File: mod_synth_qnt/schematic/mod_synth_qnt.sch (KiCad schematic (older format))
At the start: 22 parts

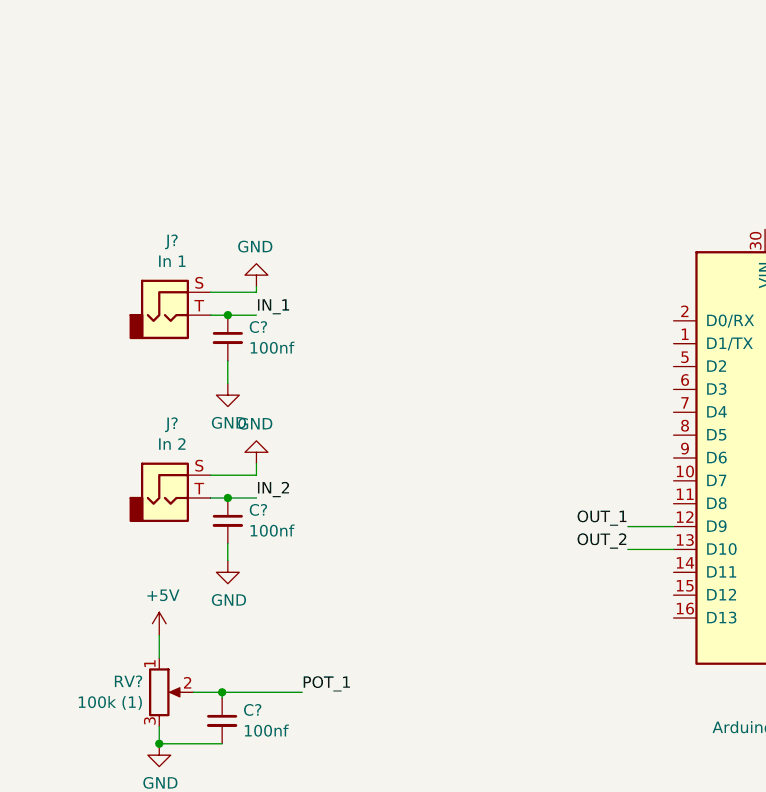
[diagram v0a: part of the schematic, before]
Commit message: Update schematic and code
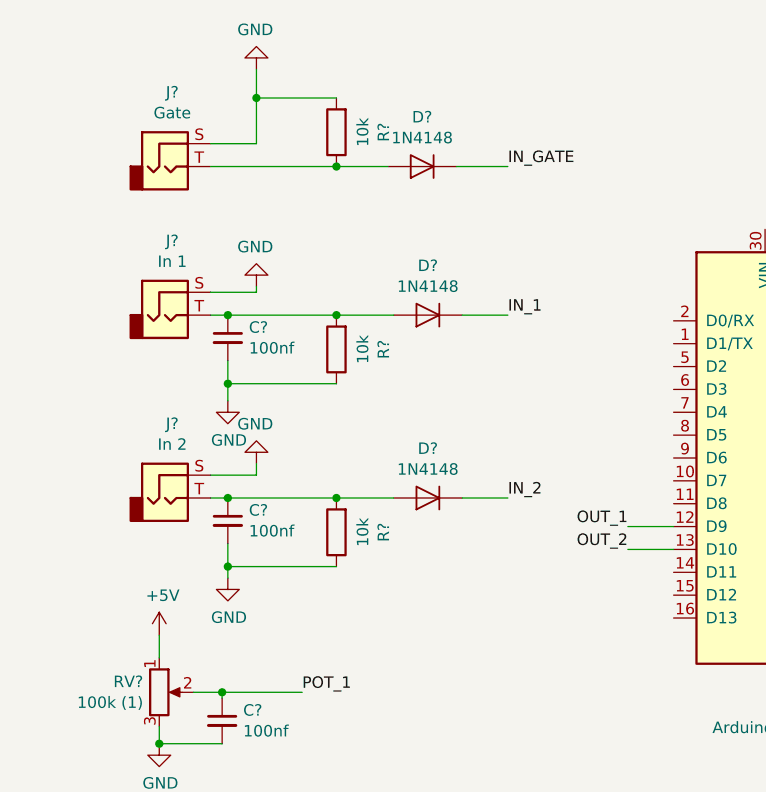
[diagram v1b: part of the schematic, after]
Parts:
- added D? (x3): 1N4148, Diode_THT:D_DO-35_SOD27_P7.62mm_Horizontal, symbol Diode:1N4148
- added J?: Gate, symbol Connector:AudioJack2
- added R? (x3): 10k, symbol Device:R
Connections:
- net GND: now also J?.S, R?.1, R?.1, R?.2
- net IN_1: now also D?.1 (K); no longer C?.1, J?.T
- net IN_2: now also D?.1 (K); no longer C?.1, J?.T
- new net: C?.1, D?.2 (A), J?.T, R?.2 (x2)
- new net: D?.2 (A), J?.T, R?.1
- new net IN_GATE: D?.1 (K)
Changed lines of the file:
@@
 	-1   0    0    -1
 $EndComp
-Text Label 3200 2300 0    50   ~ 0
+Text Label 4300 2300 0    50   ~ 0
 IN_1
-Text Label 3200 3100 0    50   ~ 0
+Text Label 4300 3100 0    50   ~ 0
 IN_2
 $Comp
@@
 Wire Wire Line
 	3200 2950 3200 3000
-Wire Wire Line
-	3200 3100 3075 3100
-Wire Wire Line
-	3200 2300 3075 2300
 Text Label 6225 2925 0    50   ~ 0
 IN_1
@@
 L power:GND #PWR?
 U 1 1 5D619ACB
-P 3075 2600
-F 0 "#PWR?" H 3075 2350 50  0001 C CNN
-F 1 "GND" H 3080 2427 50  0000 C CNN
-F 2 "" H 3075 2600 50  0001 C CNN
-F 3 "" H 3075 2600 50  0001 C CNN
-	1    3075 2600
+P 3075 2675
+F 0 "#PWR?" H 3075 2425 50  0001 C CNN
+F 1 "GND" H 3080 2502 50  0000 C CNN
+F 2 "" H 3075 2675 50  0001 C CNN
+F 3 "" H 3075 2675 50  0001 C CNN
+	1    3075 2675
 	1    0    0    -1
 $EndComp
@@
 L power:GND #PWR?
 U 1 1 5D61A0C8
-P 3075 3375
-F 0 "#PWR?" H 3075 3125 50  0001 C CNN
-F 1 "GND" H 3080 3202 50  0000 C CNN
-F 2 "" H 3075 3375 50  0001 C CNN
-F 3 "" H 3075 3375 50  0001 C CNN
-	1    3075 3375
+P 3075 3450
+F 0 "#PWR?" H 3075 3200 50  0001 C CNN
+F 1 "GND" H 3080 3277 50  0000 C CNN
+F 2 "" H 3075 3450 50  0001 C CNN
+F 3 "" H 3075 3450 50  0001 C CNN
+	1    3075 3450
 	1    0    0    -1
 $EndComp
 Wire Wire Line
 	3075 2600 3075 2500
-Wire Wire Line
-	3075 3300 3075 3375
 $Comp
 L power:GND #PWR?
@@
 NoConn ~ 8275 5300
 NoConn ~ 8275 5200
+$Comp
+L Device:R R?
+U 1 1 5D61316C
+P 3550 2450
+F 0 "R?" V 3343 2450 50  0000 C CNN
+F 1 "10k" V 3434 2450 50  0000 C CNN
+F 2 "" V 3480 2450 50  0001 C CNN
+F 3 "~" H 3550 2450 50  0001 C CNN
+	1    3550 2450
+	-1   0    0    1
+$EndComp
+$Comp
+L Device:R R?
+U 1 1 5D6143B5
+P 3550 3250
+F 0 "R?" V 3343 3250 50  0000 C CNN
+F 1 "10k" V 3434 3250 50  0000 C CNN
+F 2 "" V 3480 3250 50  0001 C CNN
+F 3 "~" H 3550 3250 50  0001 C CNN
+	1    3550 3250
+	-1   0    0    1
+$EndComp
+Wire Wire Line
+	3075 2300 3550 2300
+Wire Wire Line
+	3550 2300 3800 2300
+Connection ~ 3550 2300
+Wire Wire Line
+	3075 3100 3550 3100
+Connection ~ 3550 3100
+Wire Wire Line
+	3550 3100 3800 3100
+Wire Wire Line
+	3550 2600 3075 2600
+Wire Wire Line
+	3075 2600 3075 2675
+Connection ~ 3075 2600
+Wire Wire Line
+	3550 3400 3075 3400
+Wire Wire Line
+	3075 3300 3075 3400
+Connection ~ 3075 3400
+Wire Wire Line
+	3075 3400 3075 3450
+$Comp
+L Connector:AudioJack2 J?
+U 1 1 5D62A188
+P 2800 1650
+F 0 "J?" H 2832 1975 50  0000 C CNN
+F 1 "Gate" H 2832 1884 50  0000 C CNN
+F 2 "" H 2800 1650 50  0001 C CNN
+F 3 "~" H 2800 1650 50  0001 C CNN
+	1    2800 1650
+	1    0    0    -1
+$EndComp
+$Comp
+L power:GND #PWR?
+U 1 1 5D62A425
+P 3200 1225
+F 0 "#PWR?" H 3200 975 50  0001 C CNN
+F 1 "GND" H 3205 1052 50  0000 C CNN
+F 2 "" H 3200 1225 50  0001 C CNN
+F 3 "" H 3200 1225 50  0001 C CNN
+	1    3200 1225
+	-1   0    0    1
+$EndComp
+Wire Wire Line
+	3000 1550 3200 1550
+Text Label 4300 1650 0    50   ~ 0
+IN_GATE
+Wire Wire Line
+	3000 1650 3550 1650
+$Comp
+L Diode:1N4148 D?
+U 1 1 5D630B6B
+P 3925 1650
+F 0 "D?" H 3925 1434 50  0000 C CNN
+F 1 "1N4148" H 3925 1525 50  0000 C CNN
+F 2 "Diode_THT:D_DO-35_SOD27_P7.62mm_Horizontal" H 3925 1475 50  0001 C CNN
+F 3 "https://assets.nexperia.com/documents/data-sheet/1N4148_1N4448.pdf" H 3925 1650 50  0001 C CNN
+	1    3925 1650
+	-1   0    0    1
+$EndComp
+$Comp
+L Diode:1N4148 D?
+U 1 1 5D631B5D
+P 3950 2300
+F 0 "D?" H 3950 2084 50  0000 C CNN
+F 1 "1N4148" H 3950 2175 50  0000 C CNN
+F 2 "Diode_THT:D_DO-35_SOD27_P7.62mm_Horizontal" H 3950 2125 50  0001 C CNN
+F 3 "https://assets.nexperia.com/documents/data-sheet/1N4148_1N4448.pdf" H 3950 2300 50  0001 C CNN
+	1    3950 2300
+	-1   0    0    1
+$EndComp
+$Comp
+L Diode:1N4148 D?
+U 1 1 5D631FDA
+P 3950 3100
+F 0 "D?" H 3950 2884 50  0000 C CNN
+F 1 "1N4148" H 3950 2975 50  0000 C CNN
+F 2 "Diode_THT:D_DO-35_SOD27_P7.62mm_Horizontal" H 3950 2925 50  0001 C CNN
+F 3 "https://assets.nexperia.com/documents/data-sheet/1N4148_1N4448.pdf" H 3950 3100 50  0001 C CNN
+	1    3950 3100
+	-1   0    0    1
+$EndComp
+$Comp
+L Device:R R?
+U 1 1 5D633789
+P 3550 1500
+F 0 "R?" V 3343 1500 50  0000 C CNN
+F 1 "10k" V 3434 1500 50  0000 C CNN
+F 2 "" V 3480 1500 50  0001 C CNN
+F 3 "~" H 3550 1500 50  0001 C CNN
+	1    3550 1500
+	-1   0    0    1
+$EndComp
+Connection ~ 3550 1650
+Wire Wire Line
+	3550 1650 3775 1650
+Wire Wire Line
+	4075 1650 4300 1650
+Wire Wire Line
+	4300 2300 4100 2300
+Wire Wire Line
+	4100 3100 4300 3100
+Wire Wire Line
+	3200 1225 3200 1350
+Wire Wire Line
+	3550 1350 3200 1350
+Connection ~ 3200 1350
+Wire Wire Line
+	3200 1350 3200 1550
 $EndSCHEMATC
